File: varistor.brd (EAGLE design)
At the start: 76.2 x 25.4 mm, 2 parts

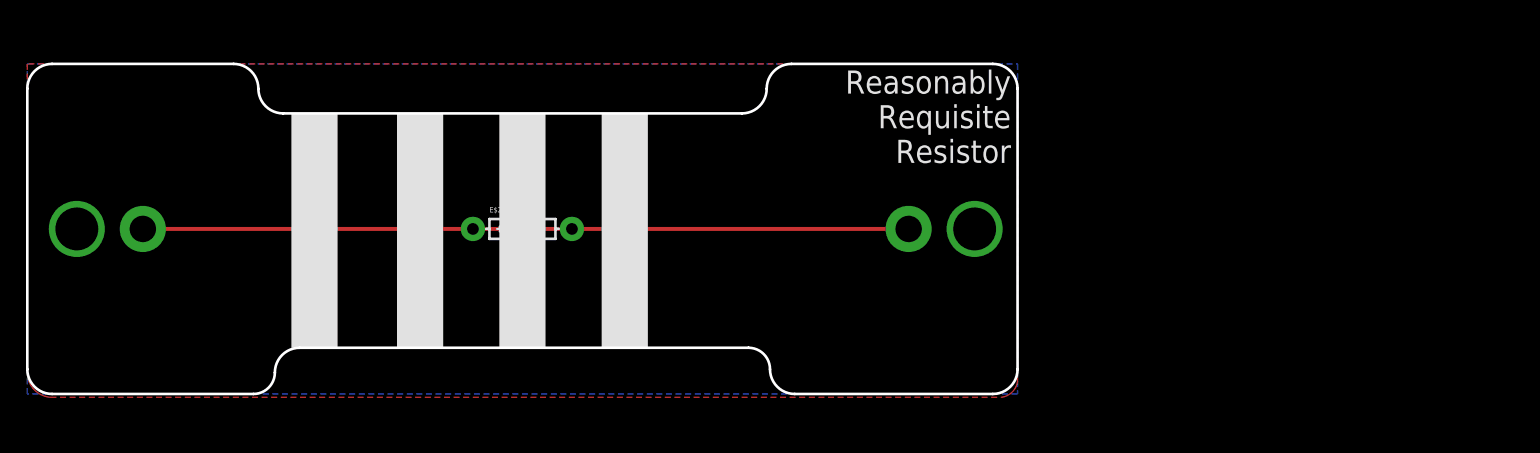
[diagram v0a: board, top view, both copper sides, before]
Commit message: confirm footprints and finalize for maker faire
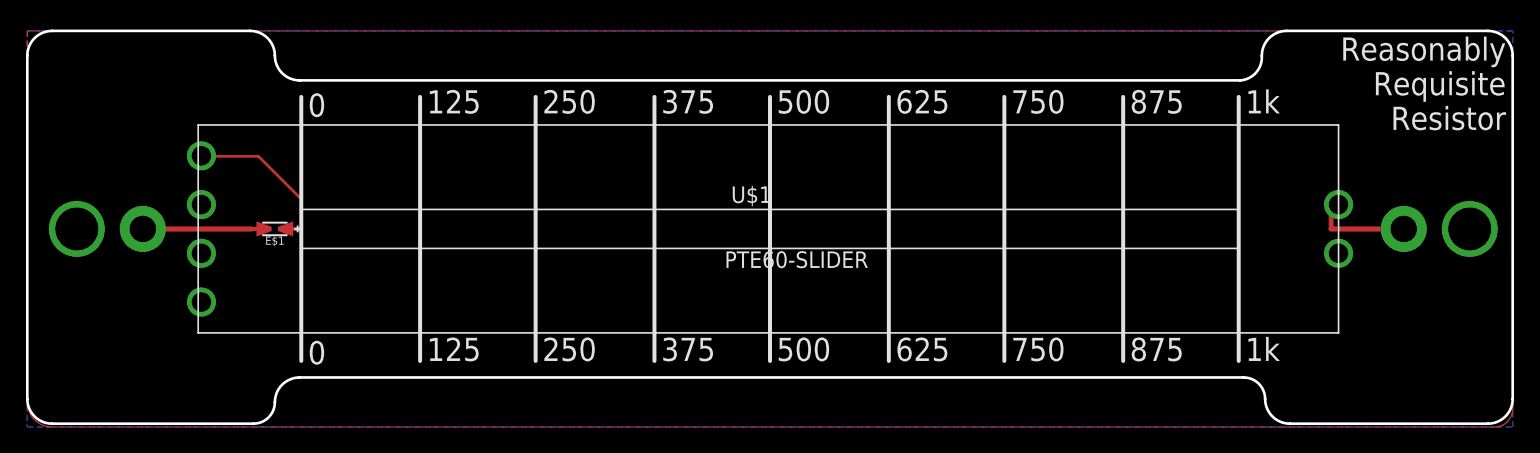
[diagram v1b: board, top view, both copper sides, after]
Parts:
- removed E$2: (no value), tekdemo:AXIAL-0.3
- added U$1: PTE60-SLIDER, lt3092:SLIDER
- moved E$1 19.1 mm to (19.1, 12.7), turned to 180 degrees
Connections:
- new net N$1: U$1.1
- new net N$2: U$1.2
- new net N$3: U$1.3
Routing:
- net S$4: track 28.7 -> 7.87 mm
- net S$3: track 28.3 -> 21.7 mm
- added copper zone on layer 16, net N$4
- removed copper zone on layer 16, net S$6
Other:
- board size 76.2 x 25.4 mm -> 114.3 x 30.2 mm
- board text added: "0"
- board text added: "125"
- board text added: "1k"
- board text added: "250"
- board text added: "375"
- board text added: "500"
- board text added: "625"
- board text added: "750"
- board text added: "875"
- board text added: "?"
- board text added: "I'm great for figuring out how resistors can change a circuit"
- board text added: "Unlike the smaller resistors, my value can change based on the slider."
- board text removed: "If you know the trick, you can read this from my colored bands!"
- board text removed: "This is my resistance value!"
- board text removed: "ohms"
